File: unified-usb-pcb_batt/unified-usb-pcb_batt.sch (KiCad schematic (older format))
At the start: 34 parts, among them J1 QI, J2 USB_C_Receptacle_USB2.0, J3 USB_Out, J4 BATT, J5 THERM, SW1 SW_SPDT, U1 SRV05-4, U2 DW01A, U3 TP4056, U4 FS8205

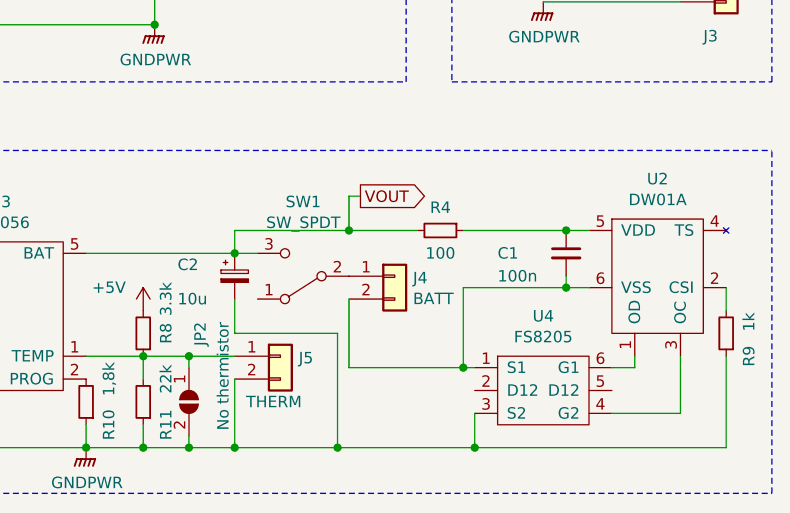
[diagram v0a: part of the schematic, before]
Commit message: started working on pcb layout
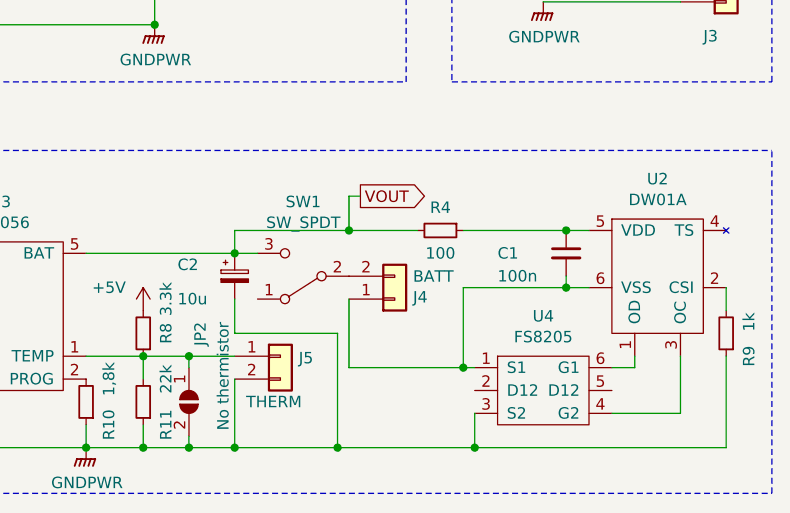
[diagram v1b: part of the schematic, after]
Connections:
- net at J4.1 (Pin_1): now also C1.2, U2.6 (VSS), U4.1 (S1); no longer SW1.2 (B)
- new net: J4.2 (Pin_2), SW1.2 (B)
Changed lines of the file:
@@
 L Connector_Generic:Conn_01x02 J4
 U 1 1 5E8AB5AC
-P 3900 3700
-F 0 "J4" H 3980 3692 50  0000 L CNN
-F 1 "BATT" H 3980 3601 50  0000 L CNN
-F 2 "Connector_JST:JST_SH_SM02B-SRSS-TB_1x02-1MP_P1.00mm_Horizontal" H 3900 3700 50  0001 C CNN
-F 3 "~" H 3900 3700 50  0001 C CNN
-	1    3900 3700
-	1    0    0    -1
+P 3900 3800
+F 0 "J4" H 3980 3792 50  0000 L CNN
+F 1 "BATT" H 3980 3701 50  0000 L CNN
+F 2 "Connector_JST:JST_SH_SM02B-SRSS-TB_1x02-1MP_P1.00mm_Horizontal" H 3900 3800 50  0001 C CNN
+F 3 "~" H 3900 3800 50  0001 C CNN
+	1    3900 3800
+	1    0    0    1
 $EndComp
 $Comp
